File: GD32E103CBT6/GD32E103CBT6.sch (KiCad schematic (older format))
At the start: 15 parts, among them J1 DBG, U1 GD32E103CBTx, Y1 16MHz

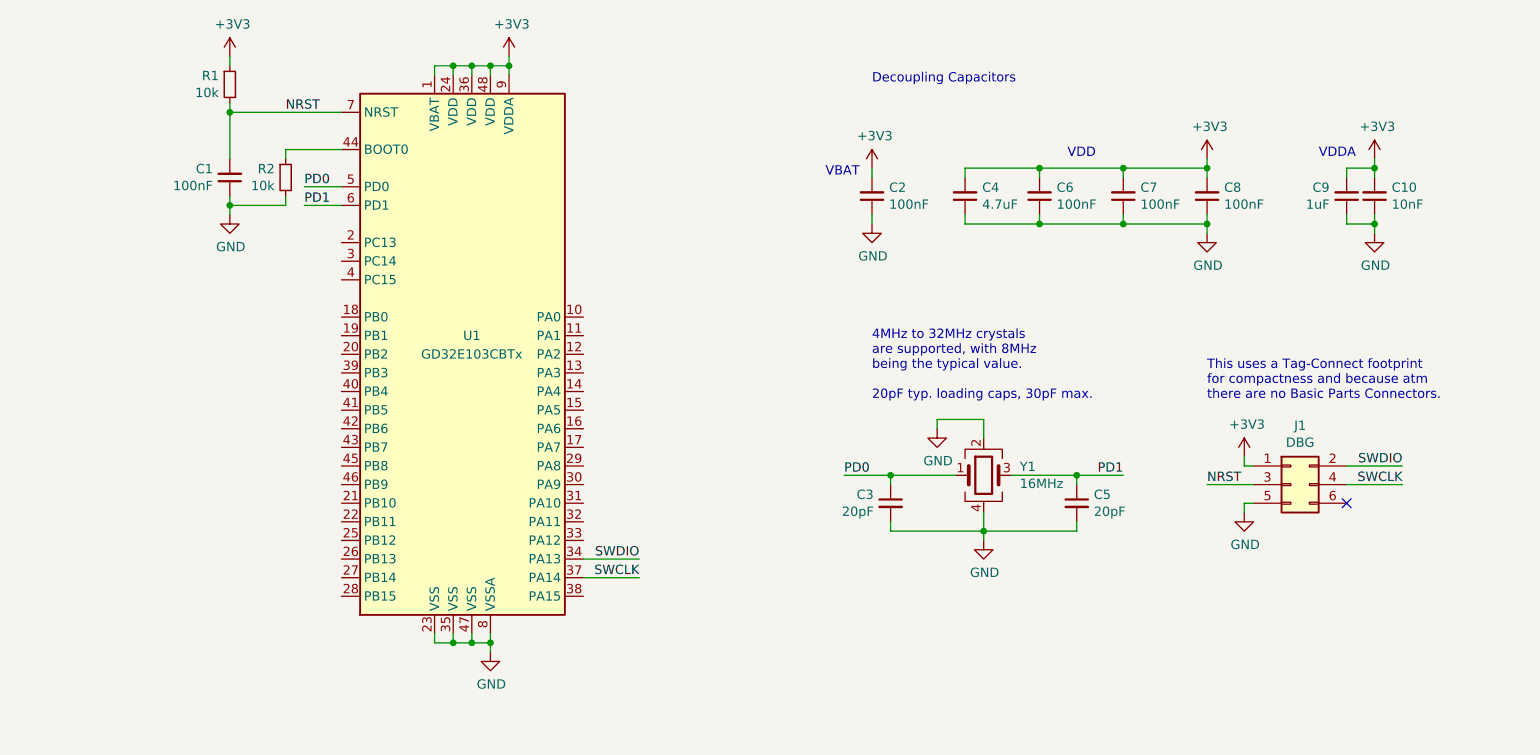
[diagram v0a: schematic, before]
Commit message: Move things around a little bit
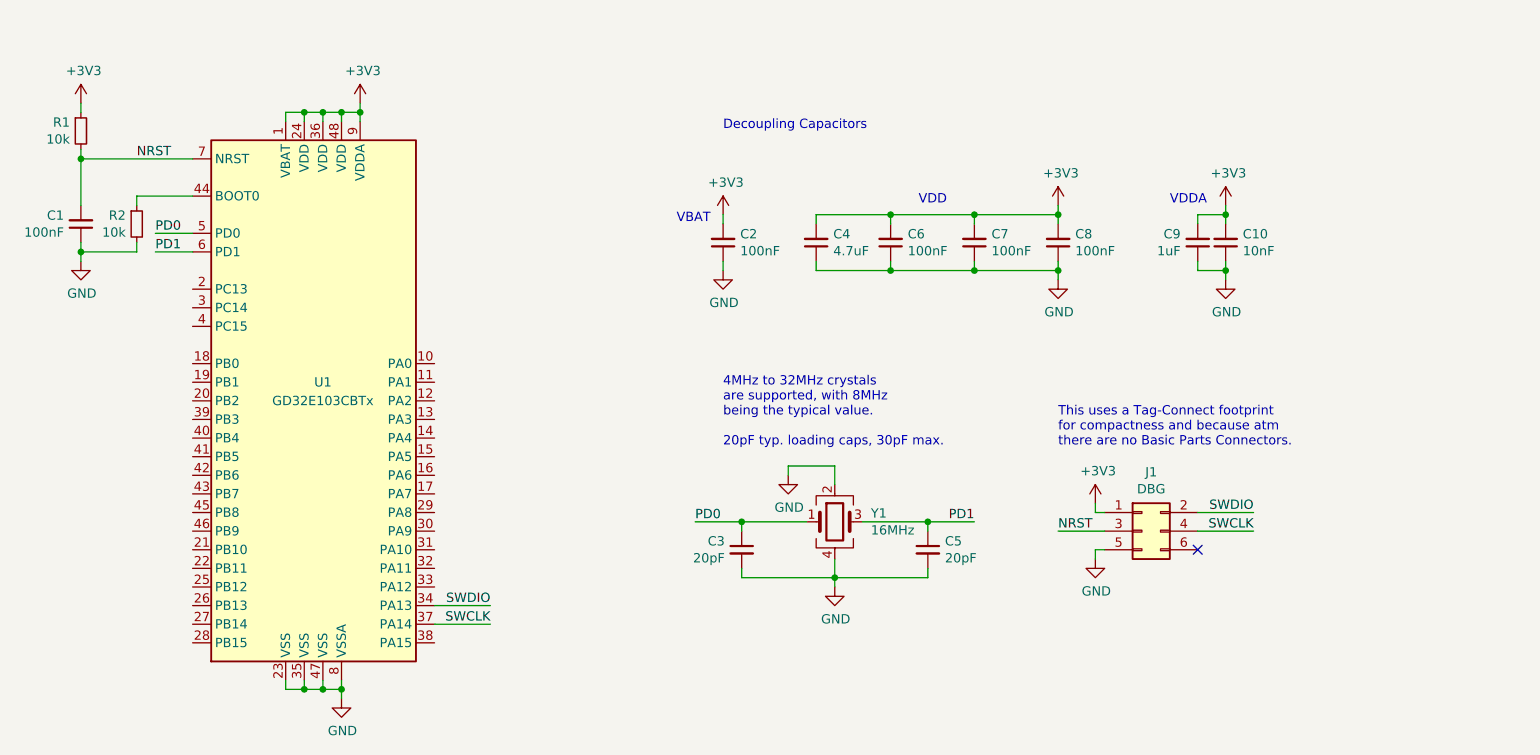
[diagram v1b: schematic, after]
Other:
- moved on the sheet: C1, C10, C2, C3, C4, C5, C6, C7, C8, C9, J1, R1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
